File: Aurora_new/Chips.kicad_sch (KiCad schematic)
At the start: 83 parts, among them J1 UJ20-C-H-C-3-SMT-TR, J16 PPPC042LFBN-RC, J3 PPPC042LFBN-RC, J36 PPPC042LFBN-RC, J41 STEMMA QT, J6 DM3AT-SF-PEJM5, U1 STM32H757BITx, U13 XBP9X-DMUS-001, U14 MS5611-01BA, U2 USBLC6-2SC6, U3 TPS2121RUXR, U5 ICM-45686, U6 ICM-40609-D, U7 BNO085, U9 MCP23017T-E_SO

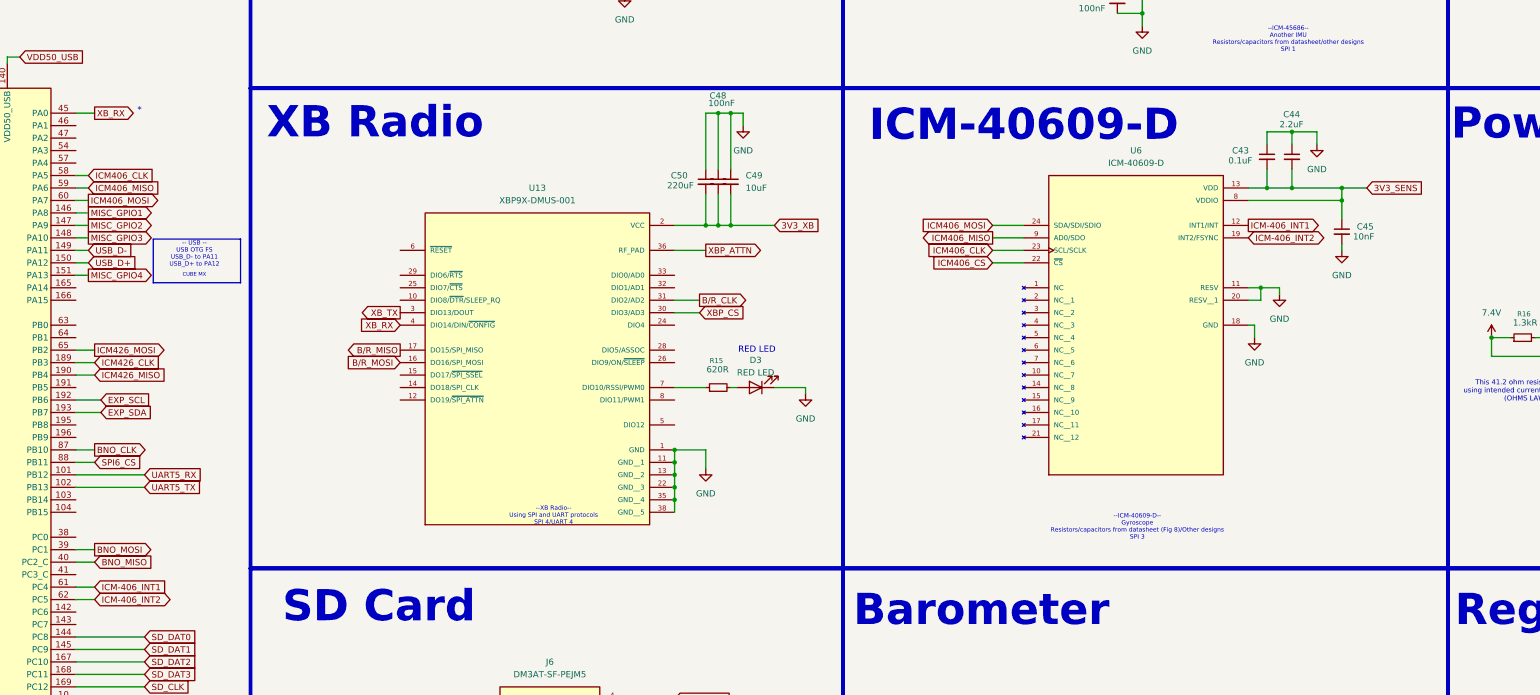
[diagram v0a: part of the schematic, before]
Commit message: undo imu switch grant got scammed
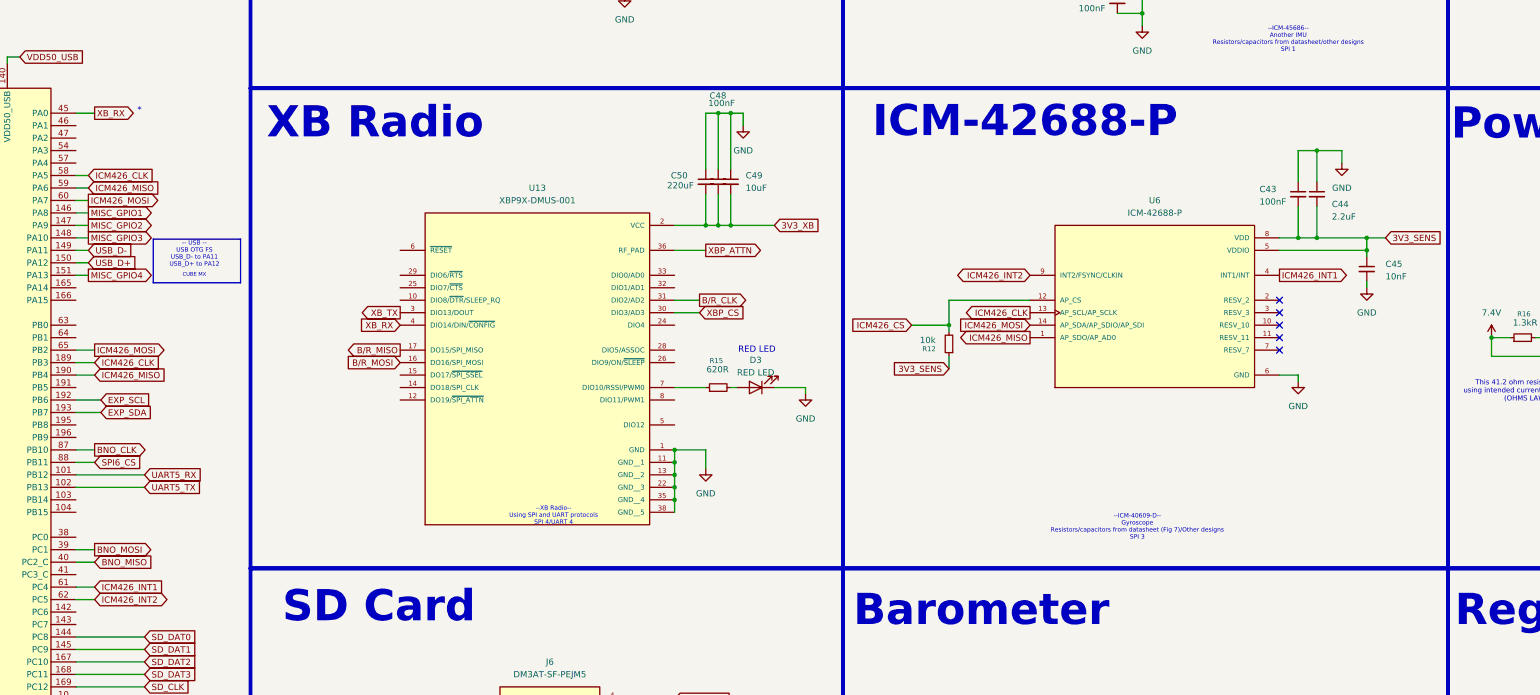
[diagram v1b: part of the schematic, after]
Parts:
- removed U6: ICM-40609-D, ICM-40609-D:XDCR_ICM-40609-D, symbol ICM-40609-D:ICM-40609-D
- added R12: 10k, Resistor_SMD:R_0805_2012Metric, symbol Device:R_Small
- added U6: ICM-42688-P, ICM-42688-P:PQFN50P300X250X97-14N, symbol ICM-42688-P:ICM-42688-P
- C43: value 0.1uF -> 100nF; footprint Capacitor_SMD:C_1206_3216Metric -> Capacitor_SMD:C_0805_2012Metric; PURCHASE-URL https://www.digikey.com/en/products/detail/murata-electroni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 -> https://www.digikey.com/en/products/detail/kyocera-avx/KGM1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; Price $0.41890 -> $0.00700
- C44, C45: footprint Capacitor_SMD:C_1206_3216Metric -> Capacitor_SMD:C_0805_2012Metric; PURCHASE-URL https://www.digikey.com/en/products/detail/murata-electroni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 -> https://www.digikey.com/en/products/detail/kyocera-avx/KGM1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; Price $0.41890 -> $0.00700
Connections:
- net ICM406_CLK is gone; now on net ICM426_CLK: U1.58 (PA5)
- net ICM406_MISO is gone; now on net ICM426_MISO: U1.59 (PA6)
- net ICM406_MOSI is gone; now on net ICM426_MOSI: U1.60 (PA7)
- net 3V3_SENS: now also R12.1, U6.5 (VDDIO), U6.8 (VDD)
- net GND: now also U6.6 (GND)
- net ICM426_CLK: now also U6.13 (AP_SCL/AP_SCLK)
- net ICM426_CS: now also R12.2, U6.12 (AP_CS)
- net ICM426_MISO: now also U6.1 (AP_SDO/AP_AD0)
- net ICM426_MOSI: now also U6.14 (AP_SDA/AP_SDIO/AP_SDI)
- net ICM-406_INT1 renamed ICM426_INT1
- net ICM426_INT1: now also U6.4 (INT1/INT)
- net ICM-406_INT2 renamed ICM426_INT2
- net ICM426_INT2: now also U6.9 (INT2/FSYNC/CLKIN)
- no-connect marks 22 -> 27
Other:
- note added: "--ICM-40609-D-- Gyroscope Resistors/capacitors from datasheet (Fig 7)/Other designs SPI 3"
- note added: "ICM-42688-P"
- note removed: "--ICM-40609-D-- Gyroscope Resistors/capacitors from datasheet (Fig 8)/Other designs SPI 3"
- note removed: "ICM-40609-D"
